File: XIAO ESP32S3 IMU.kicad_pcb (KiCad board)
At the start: 2 copper layers, 19.5 x 19.3 mm, 8 parts, among them J1 Pins1_7, J2 Pins8_14, U2 MPU-9250

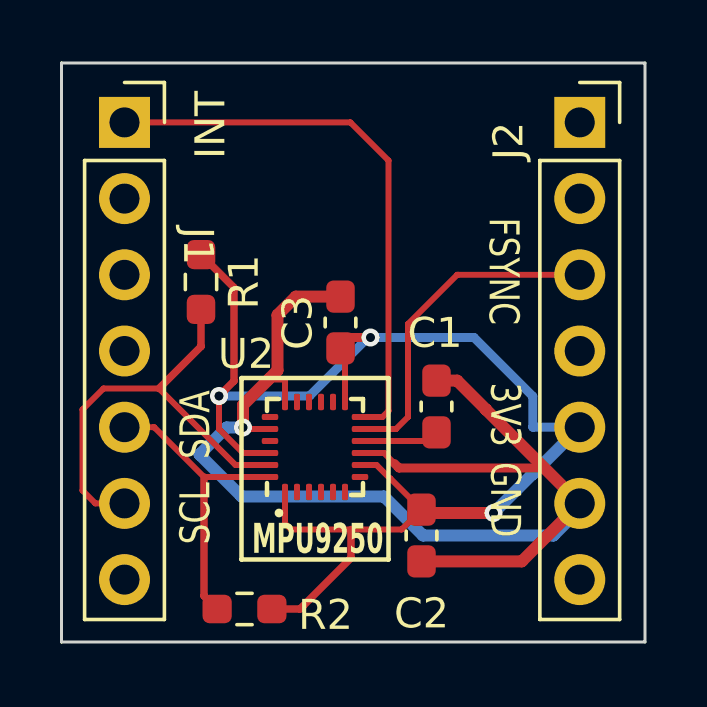
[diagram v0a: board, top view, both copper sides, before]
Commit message: gerber generation
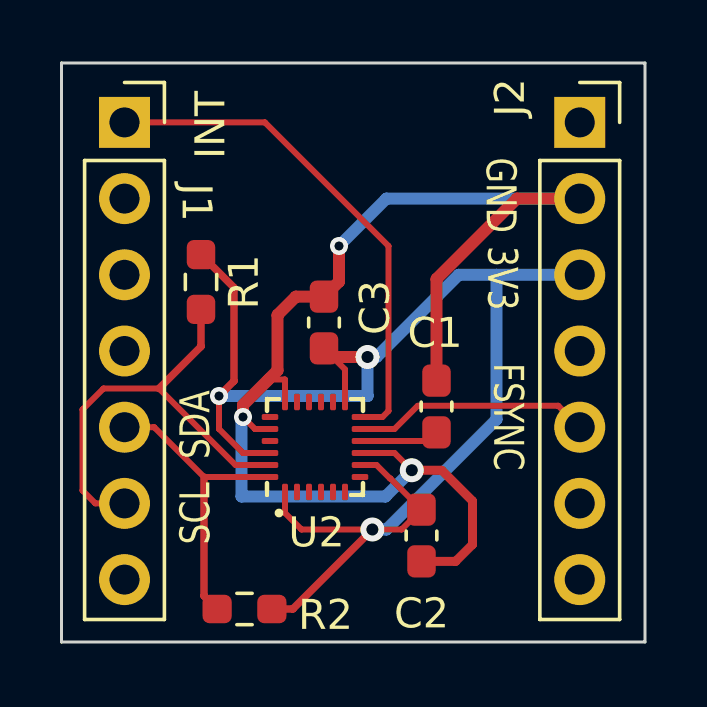
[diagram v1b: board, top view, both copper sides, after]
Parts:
- moved C3 0.55 mm to (134.6, 66.8)
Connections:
- J2 pad 2: unconnected-(J2-Pin_2-Pad2) -> GND
- J2 pad 3: /FSYNC -> /3V3
- J2 pad 5: /3V3 -> /FSYNC
- J2 pad 6: GND -> unconnected-(J2-Pin_6-Pad6)
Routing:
- net /3V3: track 45.6 -> 50.0 mm
- net /FSYNC: track 11.3 -> 7.94 mm
- net /INT: track 18.7 -> 17.0 mm
- net GND: track 43.9 -> 44.4 mm, vias 1 -> 3
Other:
- board text removed: "MPU9250"
